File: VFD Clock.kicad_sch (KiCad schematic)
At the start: 37 parts, among them J2 Mode Button, J3 Up Button, J4 Down Button, J5 Select Button, U1 74HC595, U10 74HC595, U11 UDN2981A, U12 Minute Right, U13 74HC595, U14 UDN2981A, U15 Second Left, U16 74HC595, U17 UDN2981A, U18 Second Right, U19 XL6009 Module, U2 UDN2981A, U20 LM2596 Module, U21 DS3231 Module, U3 Hour Left, U4 74HC595, U5 UDN2981A, U6 Hour Right, U7 74HC595, U8 UDN2981A, U9 Minute Left

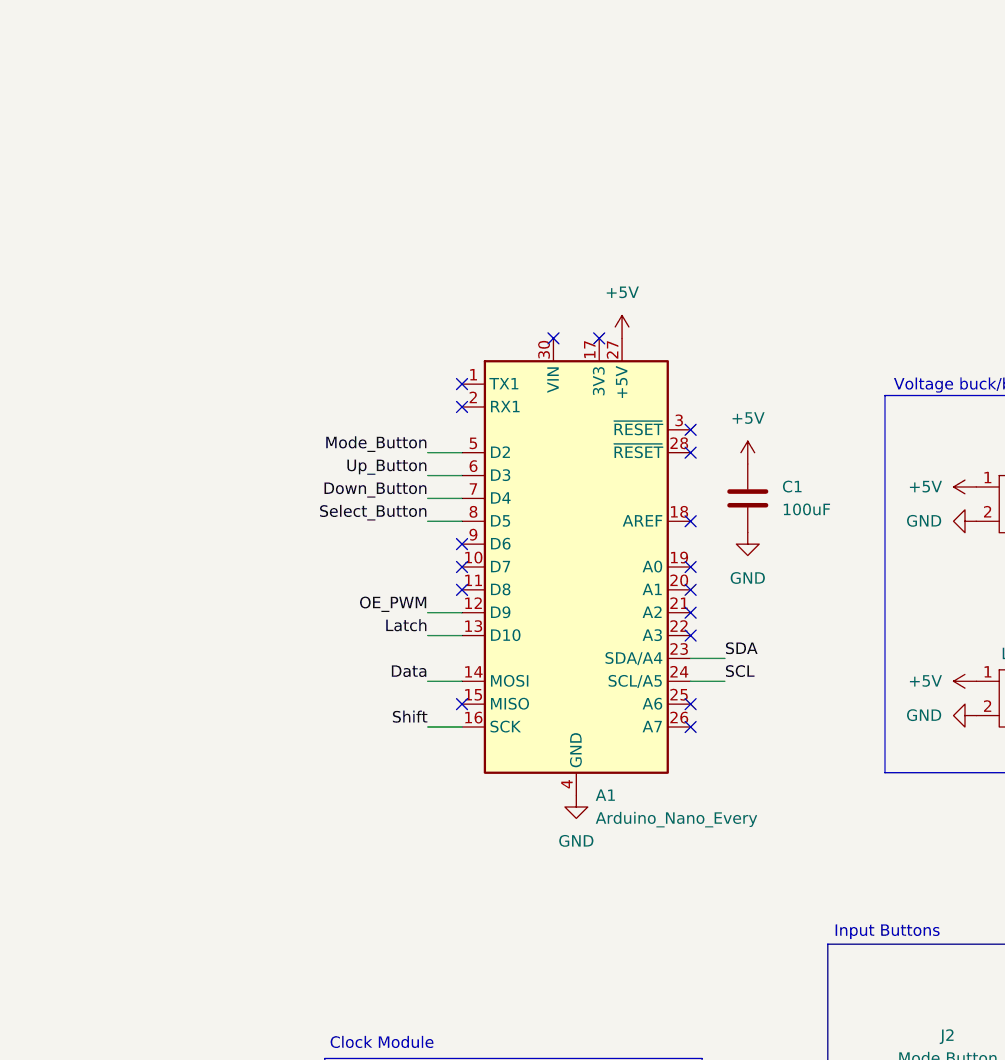
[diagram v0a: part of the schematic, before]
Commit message: checkpoint
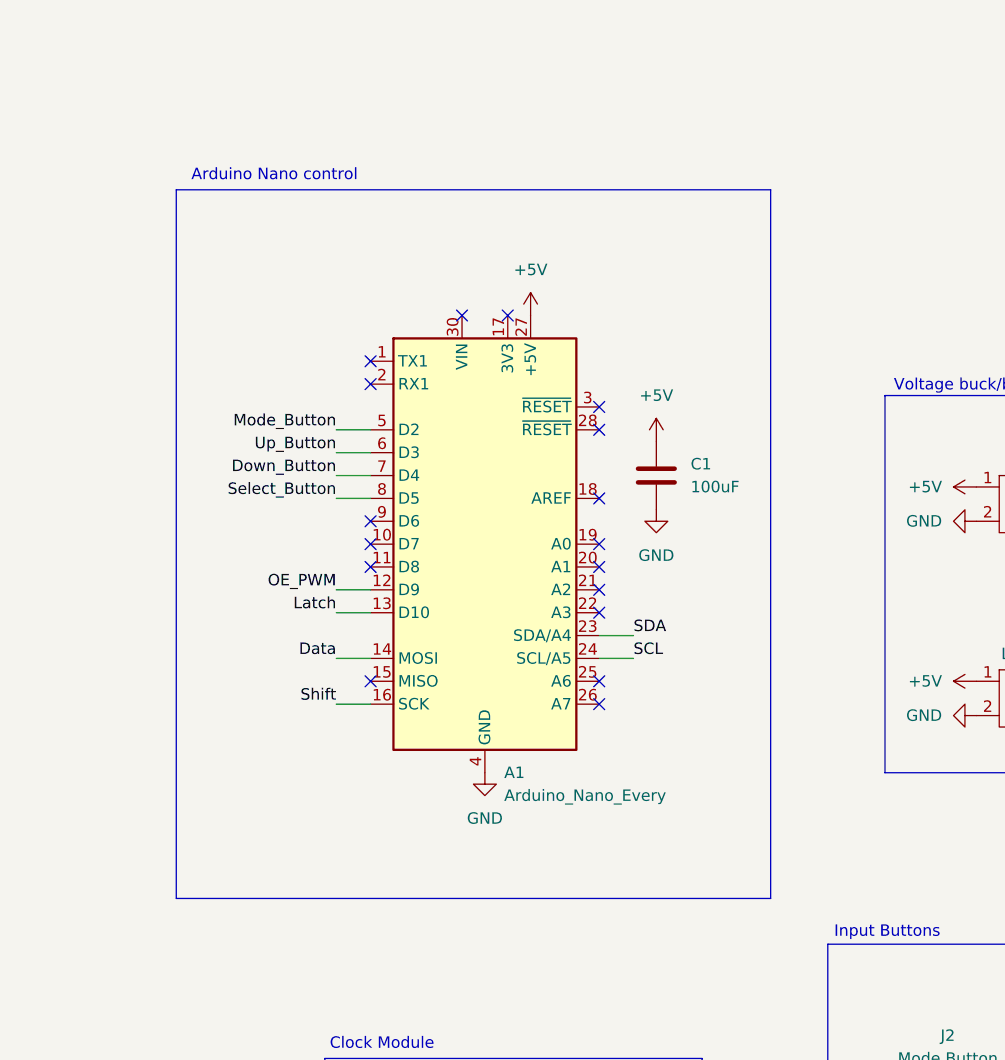
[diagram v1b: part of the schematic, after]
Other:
- note added: "Arduino Nano control"
- moved on the sheet: A1, C1
